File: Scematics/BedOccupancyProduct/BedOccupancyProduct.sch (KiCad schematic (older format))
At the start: 6 parts

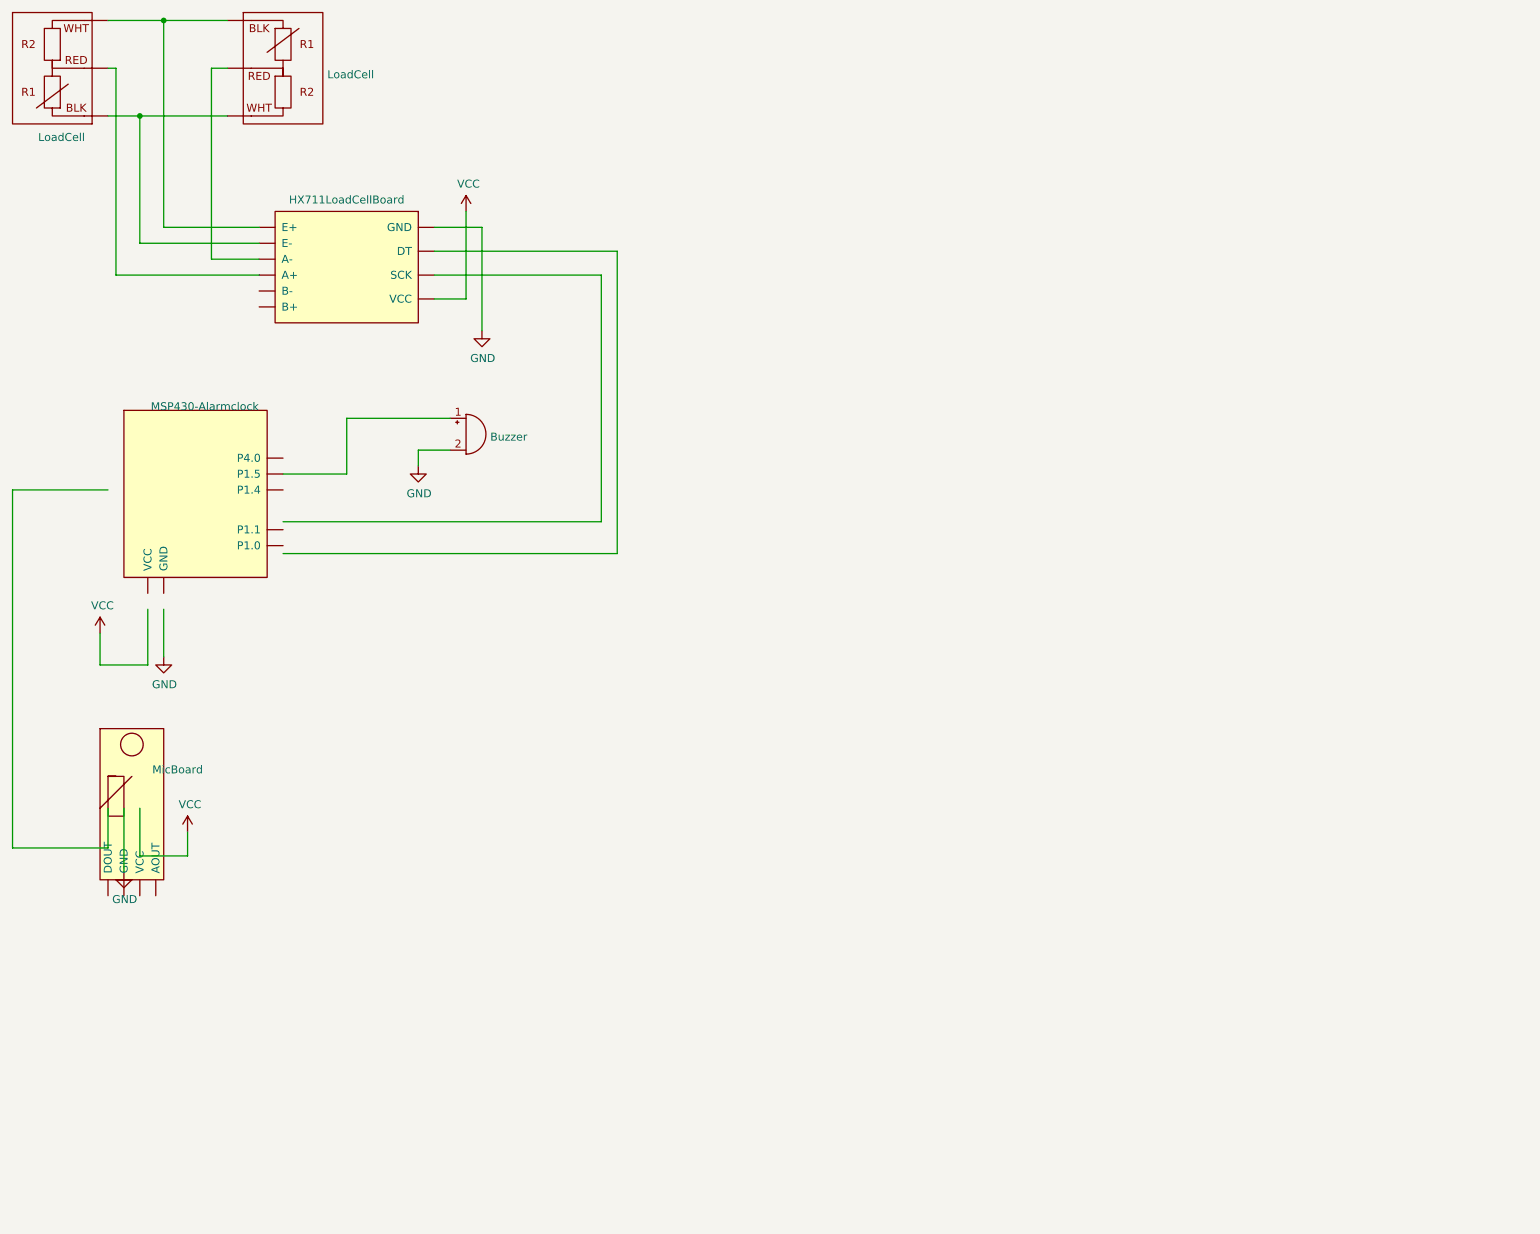
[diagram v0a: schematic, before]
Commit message: schematc update
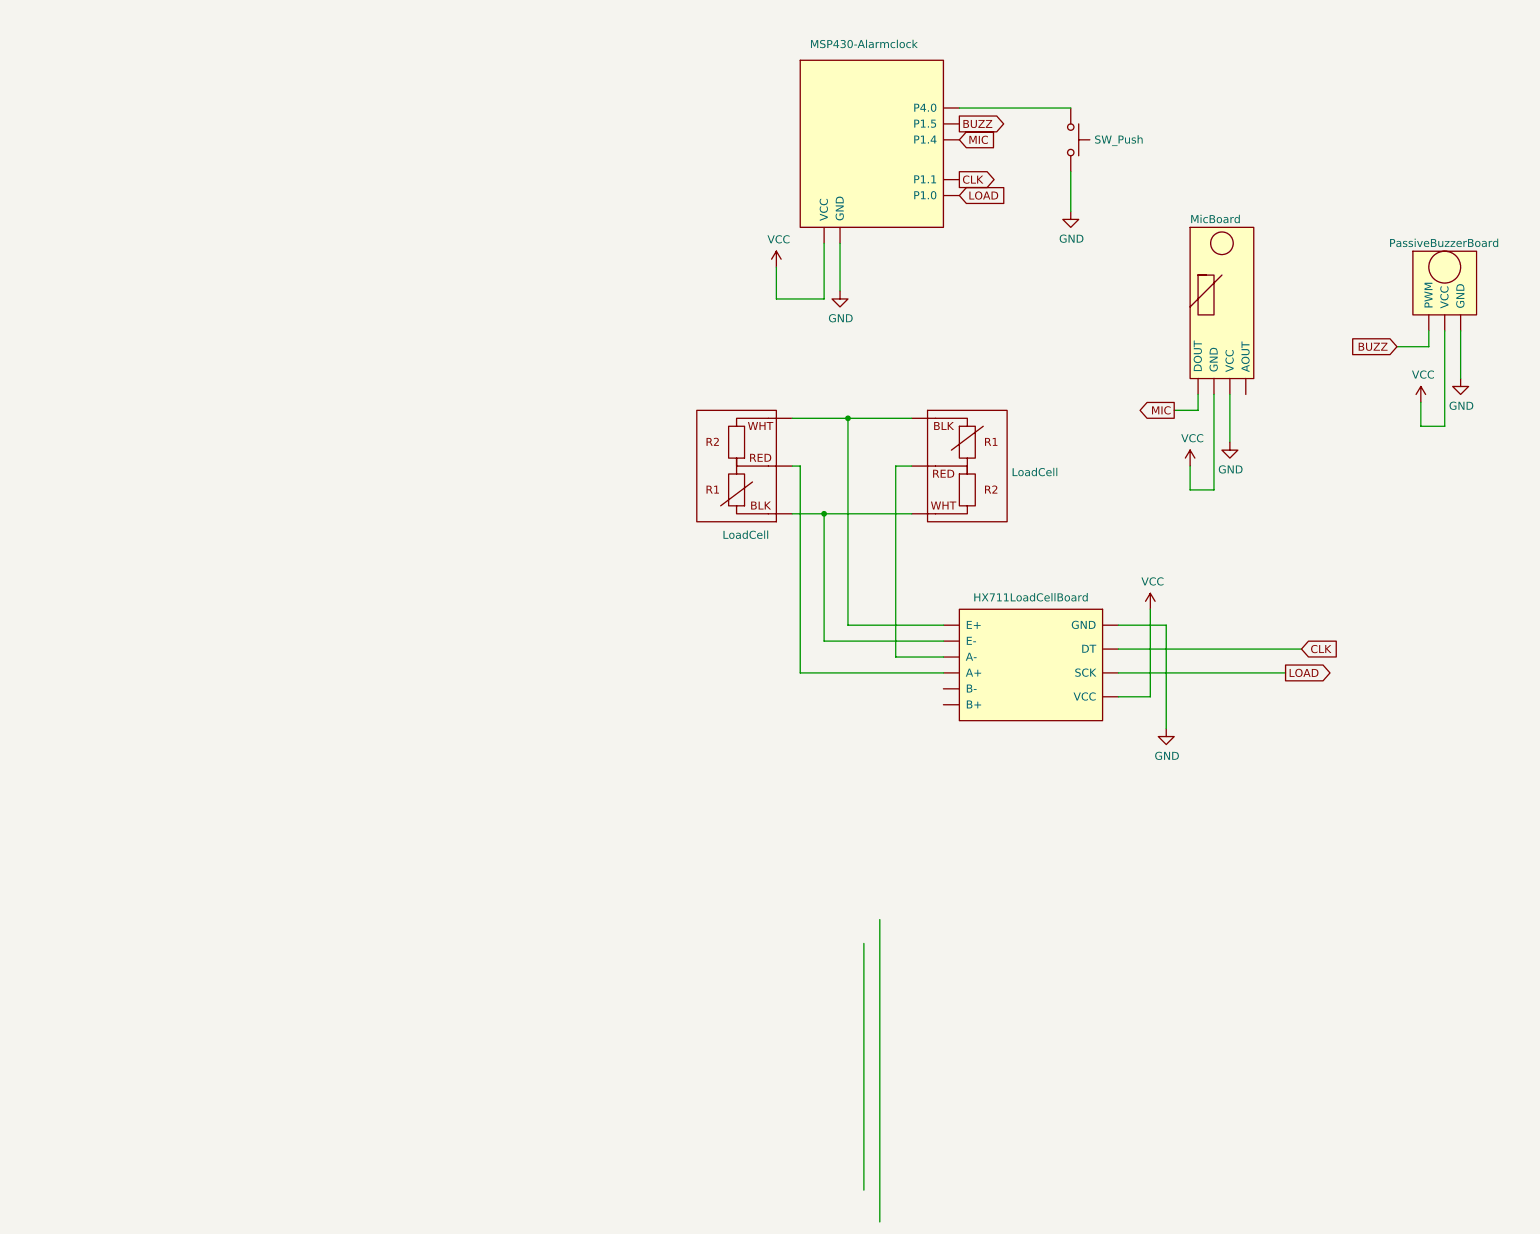
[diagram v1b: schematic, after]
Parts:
- removed BZ?: Buzzer, symbol Device:Buzzer
- added SW?: SW_Push, symbol Switch:SW_Push
- added U?: PassiveBuzzerBoard, symbol alarmclocksystem:PassiveBuzzerBoard
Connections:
- net labels added: BUZZ, CLK, LOAD, MIC
- wire segments 41 -> 40
